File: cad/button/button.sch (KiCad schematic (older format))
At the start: 30 parts, among them J1 uSD_SPI, J2 SWD, Q1 DMC2038LVT, SW1 Button, U1 STM32L072KZTx, U2 PAM8302AAS

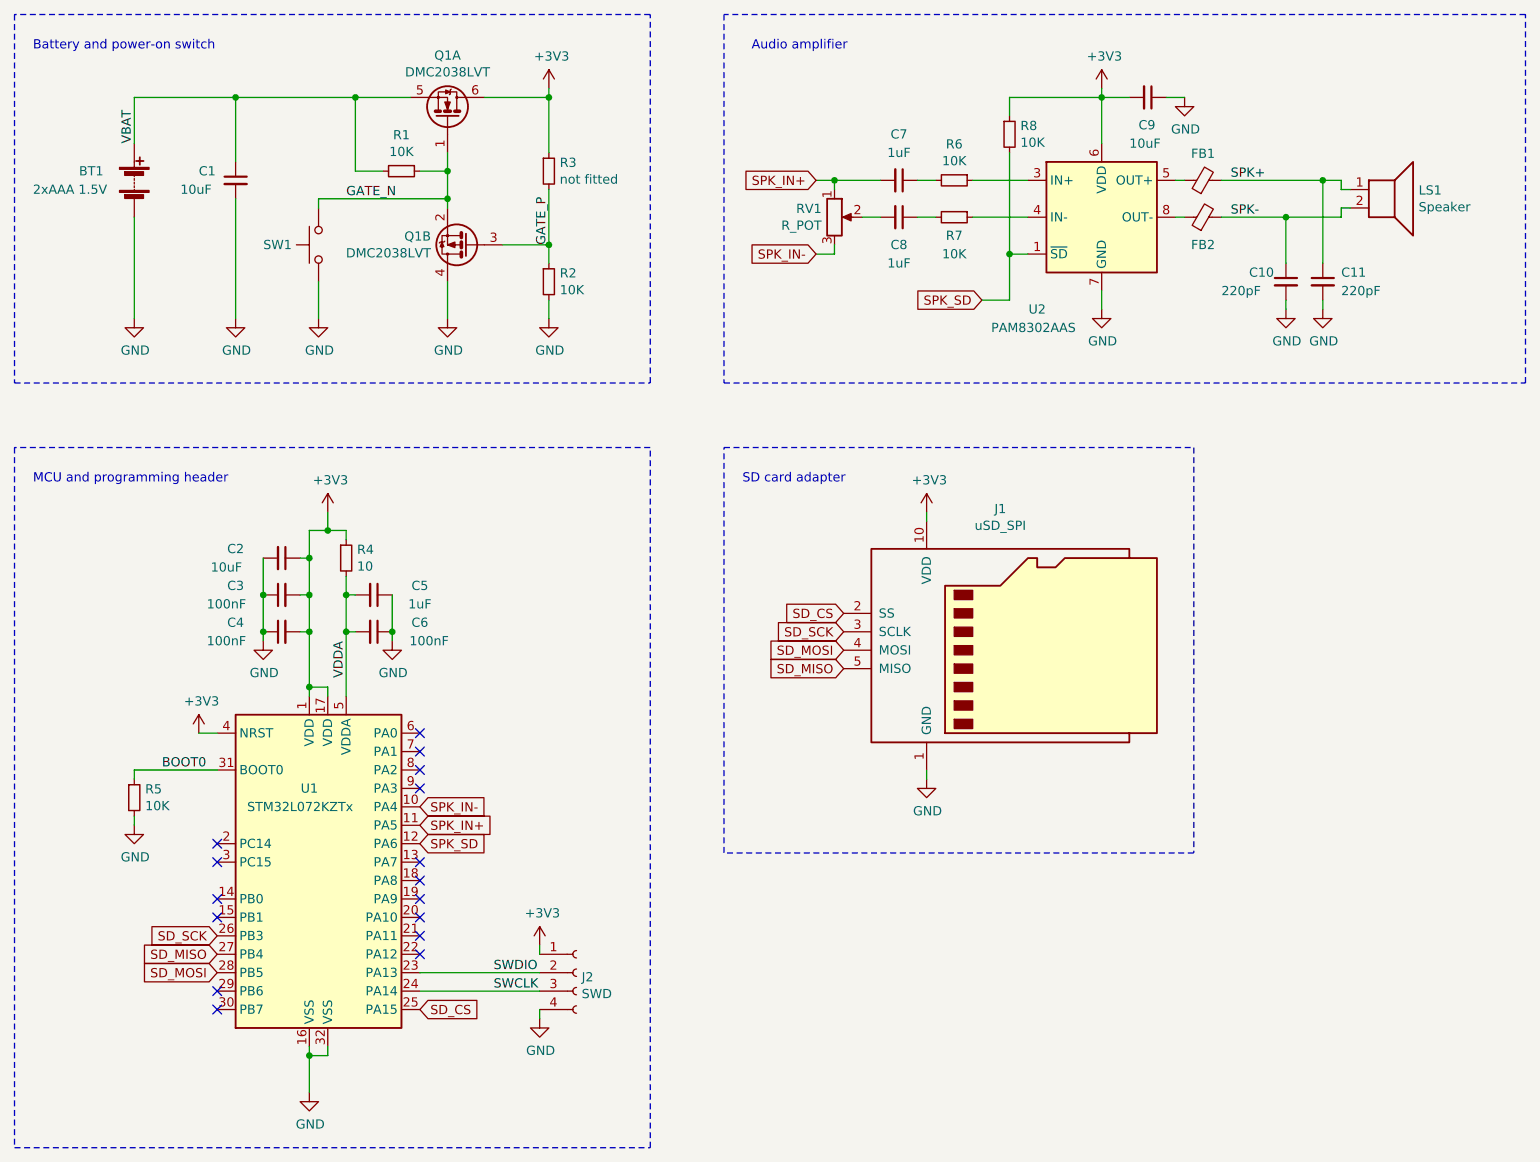
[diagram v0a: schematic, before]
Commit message: update with help from Enno
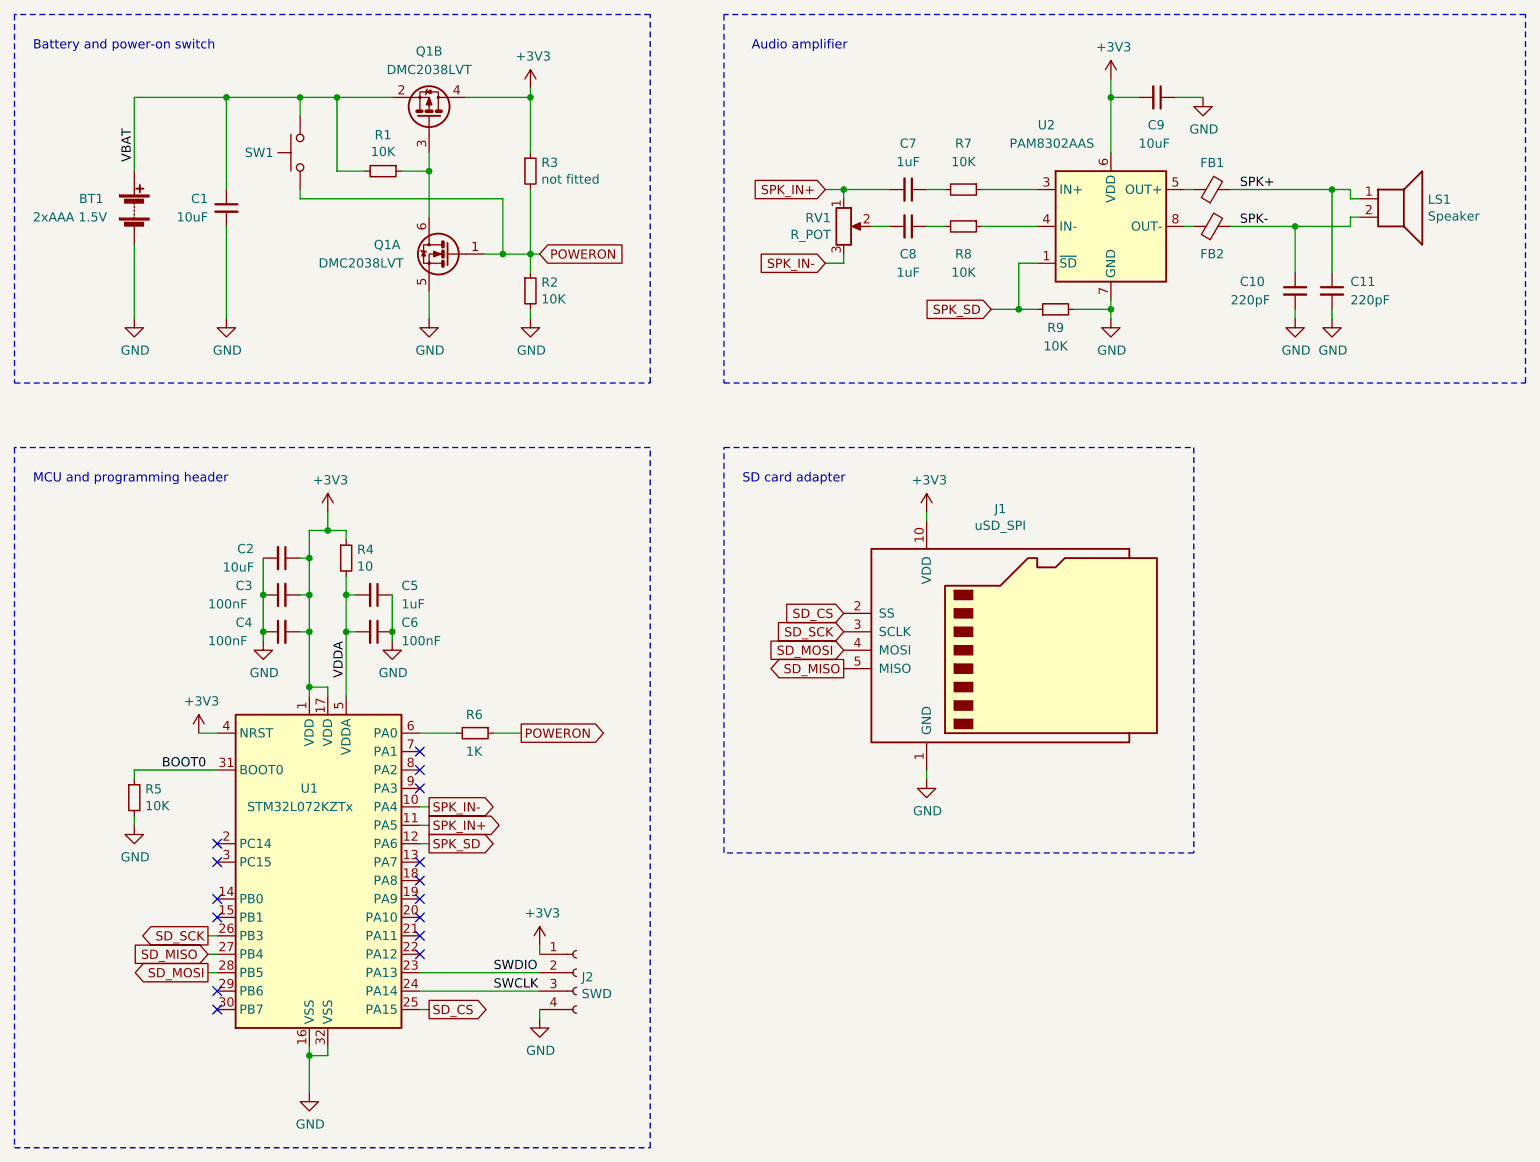
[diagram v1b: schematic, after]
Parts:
- added R6: 1K, Resistors_SMD:R_0603_HandSoldering, symbol Device:R_Small
- SW1: footprint Buttons_Switches_THT:SW_PUSH-12mm -> custom:SW_PUSH-12mm
- renumbered R6 to R7, R7 to R8, R8 to R9
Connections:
- net +3V3: now also Q1.4 (D); no longer Q1.6 (D), R9.1
- net GND: now also Q1.5 (S), R9.2; no longer Q1.4 (D), SW1.2
- net SPK_SD: now also R9.1; no longer R9.2
- net VBAT: now also Q1.2 (S), SW1.1; no longer Q1.5 (S)
- net at U1.6 (PA0): now also R6.2
- removed net GATE_N: Q1.1 (G), Q1.2 (S), R1.1, SW1.1
- net GATE_P renamed POWERON
- net POWERON: now also Q1.1 (G), SW1.2, R6.1; no longer Q1.3 (G)
- new net: Q1.3 (G), Q1.6 (D), R1.1
- no-connect marks 16 -> 15
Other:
- moved on the sheet: BT1, C1, C10, C11, C7, C8, C9, FB1, FB2, LS1, Q1A, Q1B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
